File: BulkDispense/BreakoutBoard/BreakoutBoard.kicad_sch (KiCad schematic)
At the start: 30 parts, among them J1 PS, J10 R0~R5, J11 WL1, J12 WL2, J13 DigitalOUT 0~3, J14 DigitalOUT 4~7, J15 WB1, J16 WB2, J17 AnalogIOs, J18 WB-MV1&2, J19 WB-MV3&4, J2 MV1&2, J20 FS1, J21 FS2~FS4, J22 WB-MV5&6, J24 LDS, J3 MV3&4, J4 RV1~4, J5 PCV, J6 FS1, J7 FS3, J8 FS2, J9 FS4

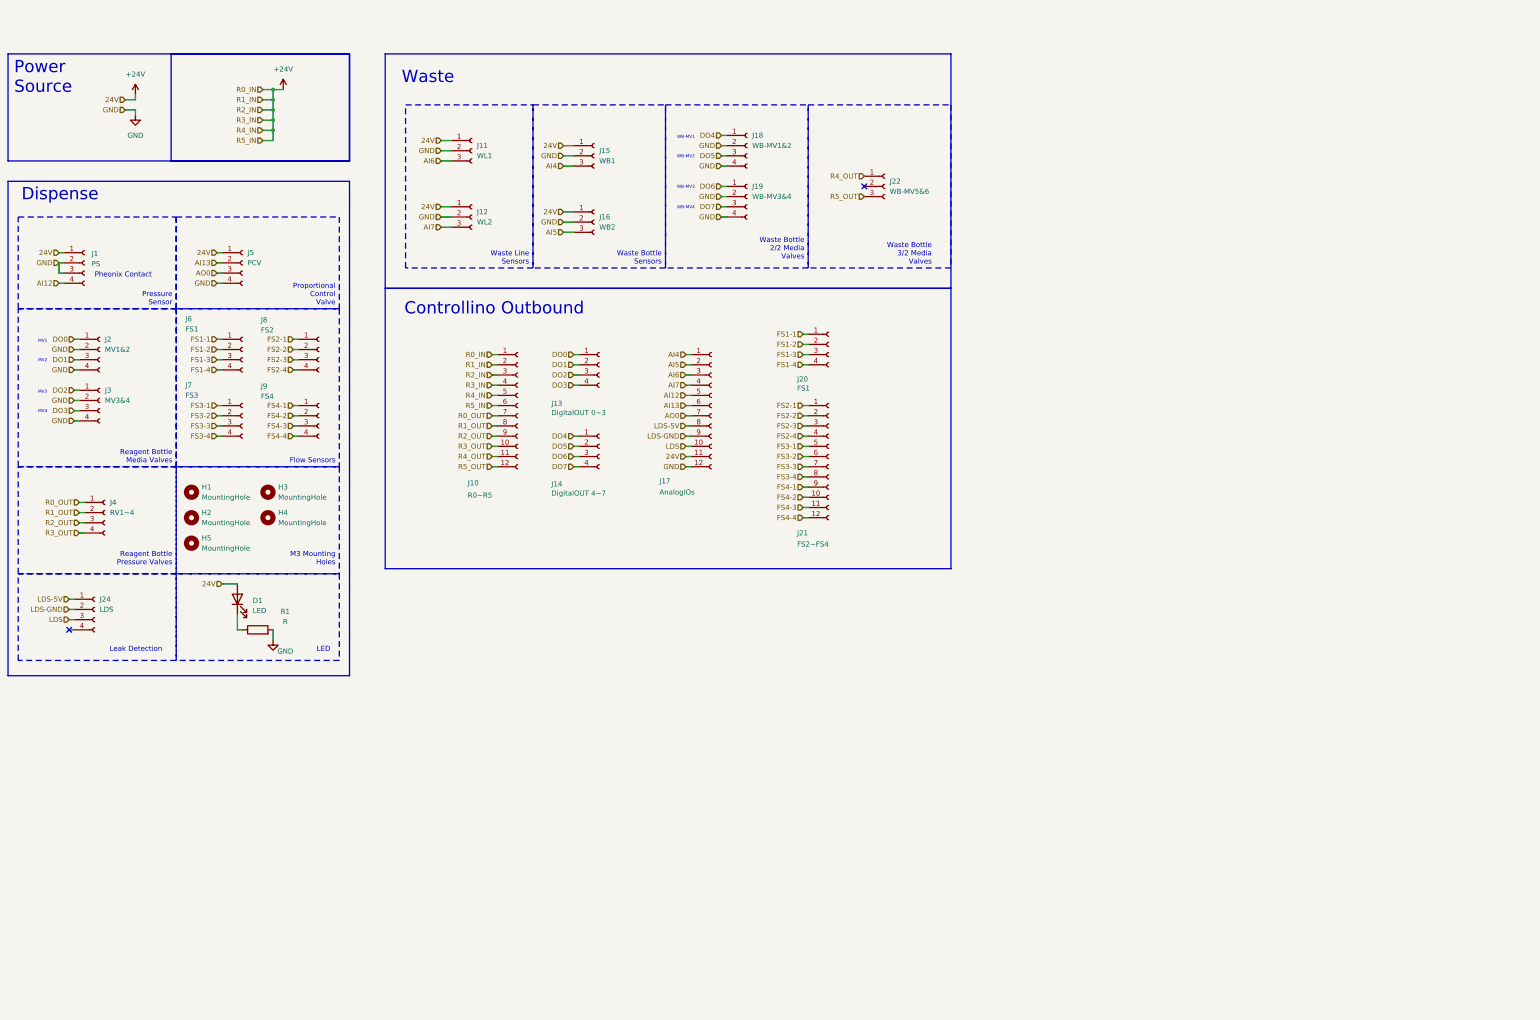
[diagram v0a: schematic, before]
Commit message: Add New Design
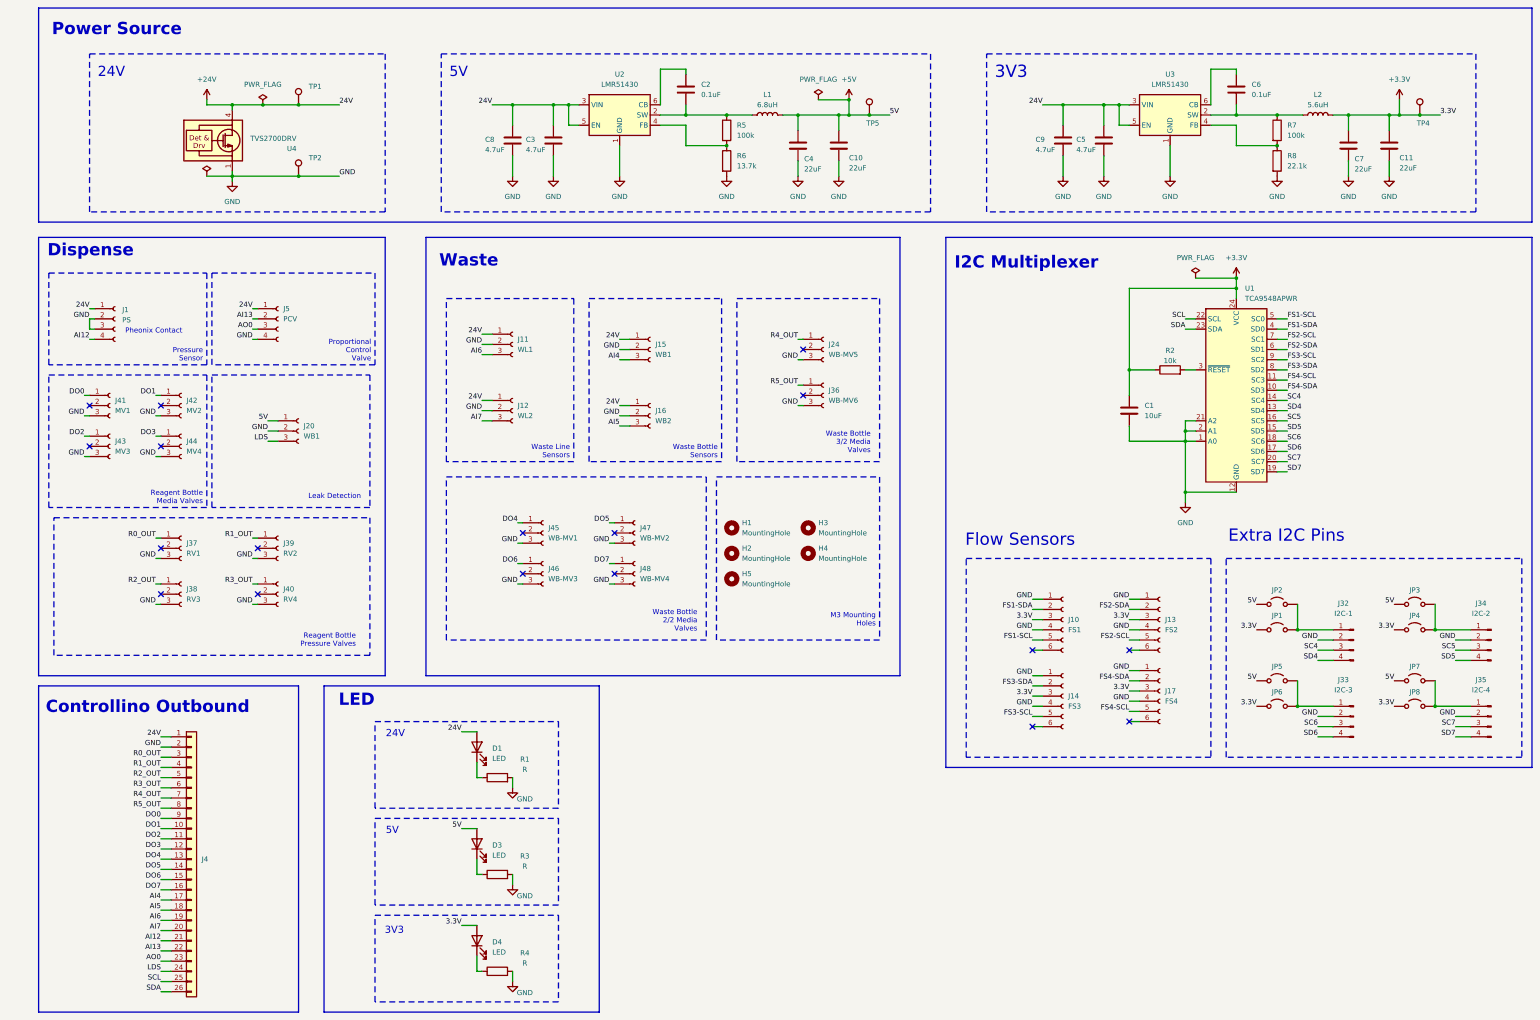
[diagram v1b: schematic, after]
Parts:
- removed J10: R0~R5, PartsLibrary:CONN_37212-62M3-003PL_3MM, symbol Connector:Conn_01x12_Socket
- removed J13: DigitalOUT 0~3, PartsLibrary:CONN_37204-62A3-004PL_3MM, symbol Connector:Conn_01x04_Socket
- removed J14: DigitalOUT 4~7, PartsLibrary:CONN_37204-62A3-004PL_3MM, symbol Connector:Conn_01x04_Socket
- removed J17: AnalogIOs, PartsLibrary:CONN_37212-62M3-003PL_3MM, symbol Connector:Conn_01x12_Socket
- removed J18: WB-MV1&2, PartsLibrary:CONN_37204-62A3-004PL_3MM, symbol Connector:Conn_01x04_Socket
- removed J19: WB-MV3&4, PartsLibrary:CONN_37204-62A3-004PL_3MM, symbol Connector:Conn_01x04_Socket
- removed J2: MV1&2, PartsLibrary:CONN_37204-62A3-004PL_3MM, symbol Connector:Conn_01x04_Socket
- removed J20, J6: FS1, PartsLibrary:CONN_37204-62A3-004PL_3MM, symbol Connector:Conn_01x04_Socket
- removed J21: FS2~FS4, PartsLibrary:CONN_37212-62M3-003PL_3MM, symbol Connector:Conn_01x12_Socket
- removed J22: WB-MV5&6, PartsLibrary:CONN_37203-62A3-003PL_3MM, symbol Connector:Conn_01x03_Socket
- removed J24: LDS, PartsLibrary:CONN_37204-62A3-004PL_3MM, symbol Connector:Conn_01x04_Socket
- removed J3: MV3&4, PartsLibrary:CONN_37204-62A3-004PL_3MM, symbol Connector:Conn_01x04_Socket
- removed J4: RV1~4, PartsLibrary:CONN_37204-62A3-004PL_3MM, symbol Connector:Conn_01x04_Socket
- removed J7: FS3, PartsLibrary:CONN_37204-62A3-004PL_3MM, symbol Connector:Conn_01x04_Socket
- removed J8: FS2, PartsLibrary:CONN_37204-62A3-004PL_3MM, symbol Connector:Conn_01x04_Socket
- removed J9: FS4, PartsLibrary:CONN_37204-62A3-004PL_3MM, symbol Connector:Conn_01x04_Socket
- added C1: 10uF, symbol Device:C
- added C10, C11, C4, C7: 22uF, symbol Device:C
- added C2, C6: 0.1uF, symbol Device:C
- added C3, C5, C8, C9: 4.7uF, symbol Device:C
- added D3, D4: LED, LED_SMD:LED_0201_0603Metric, symbol Device:LED
- added J10: FS1, symbol Connector:Conn_01x06_Socket
- added J13: FS2, symbol Connector:Conn_01x06_Socket
- added J14: FS3, symbol Connector:Conn_01x06_Socket
- added J17: FS4, symbol Connector:Conn_01x06_Socket
- added J20: WB1, PartsLibrary:CONN_37203-62A3-003PL_3MM, symbol Connector:Conn_01x03_Socket
- added J24: WB-MV5, PartsLibrary:CONN_37203-62A3-003PL_3MM, symbol Connector:Conn_01x03_Socket
- added J32: I2C-1, symbol Connector:Conn_01x04_Pin
- added J33: I2C-3, symbol Connector:Conn_01x04_Pin
- added J34: I2C-2, symbol Connector:Conn_01x04_Pin
- added J35: I2C-4, symbol Connector:Conn_01x04_Pin
- added J36: WB-MV6, PartsLibrary:CONN_37203-62A3-003PL_3MM, symbol Connector:Conn_01x03_Socket
- added J37: RV1, PartsLibrary:CONN_37203-62A3-003PL_3MM, symbol Connector:Conn_01x03_Socket
- added J38: RV3, PartsLibrary:CONN_37203-62A3-003PL_3MM, symbol Connector:Conn_01x03_Socket
- added J39: RV2, PartsLibrary:CONN_37203-62A3-003PL_3MM, symbol Connector:Conn_01x03_Socket
- added J4: Signal, PartsLibrary:CONN26_D13-ST-BK_SUL, symbol Connector_Generic:Conn_01x26
- added J40: RV4, PartsLibrary:CONN_37203-62A3-003PL_3MM, symbol Connector:Conn_01x03_Socket
- added J41: MV1, PartsLibrary:CONN_37203-62A3-003PL_3MM, symbol Connector:Conn_01x03_Socket
- added J42: MV2, PartsLibrary:CONN_37203-62A3-003PL_3MM, symbol Connector:Conn_01x03_Socket
- added J43: MV3, PartsLibrary:CONN_37203-62A3-003PL_3MM, symbol Connector:Conn_01x03_Socket
- added J44: MV4, PartsLibrary:CONN_37203-62A3-003PL_3MM, symbol Connector:Conn_01x03_Socket
- added J45: WB-MV1, PartsLibrary:CONN_37203-62A3-003PL_3MM, symbol Connector:Conn_01x03_Socket
- added J46: WB-MV3, PartsLibrary:CONN_37203-62A3-003PL_3MM, symbol Connector:Conn_01x03_Socket
- added J47: WB-MV2, PartsLibrary:CONN_37203-62A3-003PL_3MM, symbol Connector:Conn_01x03_Socket
- added J48: WB-MV4, PartsLibrary:CONN_37203-62A3-003PL_3MM, symbol Connector:Conn_01x03_Socket
- added JP1, JP2, JP3, JP4, JP5, JP6, JP7, JP8: Jumper_2_Open, Connector_PinHeader_1.00mm:PinHeader_1x02_P1.00mm_Vertical, symbol Jumper:Jumper_2_Open
- added L1: 6.8uH, symbol Device:L
- added L2: 5.6uH, symbol Device:L
- added R2: 10k, symbol Device:R
- added R3, R4: R, Resistor_SMD:R_0805_2012Metric, symbol Device:R
- added R5, R7: 100k, symbol Device:R
- added R6: 13.7k, symbol Device:R
- added R8: 22.1k, symbol Device:R
- added TP1, TP2, TP4, TP5: TestPoint, symbol Connector:TestPoint
- added U1: TCA9548APWR, Package_SO:TSSOP-24_4.4x7.8mm_P0.65mm, symbol Interface_Expansion:TCA9548APWR
- added U2, U3: LMR51430, Package_TO_SOT_SMD:SOT-23-6, symbol Regulator_Switching:LMR51430
- added U4: TVS2700DRV, Package_SON:WSON-6-1EP_2x2mm_P0.65mm_EP1x1.6mm, symbol Power_Protection:TVS2700DRV
- D1: footprint LED_SMD:LED_1206_3216Metric -> LED_SMD:LED_0201_0603Metric
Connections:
- net +24V: now also C3.1, C5.1, C8.1, C9.1, J4.1 (Pin_1), TP1.1, U2.3 (VIN), U2.5 (EN), U3.3 (VIN), U3.5 (EN), U4.4 (IN), U4.5 (IN), U4.6 (IN)
- net AI12: now also J4.21 (Pin_21)
- net AI13: now also J4.22 (Pin_22)
- net AI4: now also J4.17 (Pin_17)
- net AI5: now also J4.18 (Pin_18)
- net AI6: now also J4.19 (Pin_19)
- net AI7: now also J4.20 (Pin_20)
- net AO0: now also J4.23 (Pin_23)
- net DO0: now also J4.9 (Pin_9), J41.1 (Pin_1)
- net DO1: now also J4.10 (Pin_10), J42.1 (Pin_1)
- net DO2: now also J4.11 (Pin_11), J43.1 (Pin_1)
- net DO3: now also J4.12 (Pin_12), J44.1 (Pin_1)
- net DO4: now also J4.13 (Pin_13), J45.1 (Pin_1)
- net DO5: now also J4.14 (Pin_14), J47.1 (Pin_1)
- net DO6: now also J4.15 (Pin_15), J46.1 (Pin_1)
- net DO7: now also J4.16 (Pin_16), J48.1 (Pin_1)
- net GND: now also C1.2, C10.2, C11.2, C3.2, C4.2, C5.2, C7.2, C8.2, C9.2, J10.1 (Pin_1), J10.4 (Pin_4), J13.1 (Pin_1), J13.4 (Pin_4), J14.1 (Pin_1), J14.4 (Pin_4), J17.1 (Pin_1), J17.4 (Pin_4), J20.2 (Pin_2), J24.3 (Pin_3), J32.2 (Pin_2), J33.2 (Pin_2), J34.2 (Pin_2), J35.2 (Pin_2), J36.3 (Pin_3), J37.3 (Pin_3), J38.3 (Pin_3), J39.3 (Pin_3), J4.2 (Pin_2), J40.3 (Pin_3), J41.3 (Pin_3), J42.3 (Pin_3), J43.3 (Pin_3), J44.3 (Pin_3), J45.3 (Pin_3), J46.3 (Pin_3), J47.3 (Pin_3), J48.3 (Pin_3), R3.2, R4.2, R6.2, R8.2, TP2.1, U1.1 (A0), U1.12 (GND), U1.2 (A1), U1.21 (A2), U2.1 (GND), U3.1 (GND), U4.1 (GND), U4.2 (GND), U4.3 (GND), U4.7 (GND)
- net LDS: now also J20.3 (Pin_3), J4.24 (Pin_24)
- net R0_OUT: now also J37.1 (Pin_1), J4.3 (Pin_3)
- net R1_OUT: now also J39.1 (Pin_1), J4.4 (Pin_4)
- net R2_OUT: now also J38.1 (Pin_1), J4.5 (Pin_5)
- net R3_OUT: now also J4.6 (Pin_6), J40.1 (Pin_1)
- net R4_OUT: now also J24.1 (Pin_1), J4.7 (Pin_7)
- net R5_OUT: now also J36.1 (Pin_1), J4.8 (Pin_8)
- new net: J33.1 (Pin_1), JP5.2 (B), JP6.2 (B)
- new net: C2.1, U2.6 (CB)
- new net: C2.2, L1.1, R5.1, U2.2 (SW)
- new net: J35.1 (Pin_1), JP7.2 (B), JP8.2 (B)
- new net: J34.1 (Pin_1), JP3.2 (B), JP4.2 (B)
- new net: J32.1 (Pin_1), JP1.2 (B), JP2.2 (B)
- new net: C6.1, U3.6 (CB)
- new net: C6.2, L2.1, R7.1, U3.2 (SW)
- new net: D4.1 (K), R4.1
- new net: R7.2, R8.1, U3.4 (FB)
- new net: R2.2, U1.3 (~{RESET})
- new net: R5.2, R6.1, U2.4 (FB)
- new net: D3.1 (K), R3.1
- new net +3.3V: C1.1, C11.1, C7.1, D4.2 (A), J10.3 (Pin_3), J13.3 (Pin_3), J14.3 (Pin_3), J17.3 (Pin_3), JP1.1 (A), JP4.1 (A), JP6.1 (A), JP8.1 (A), L2.2, R2.1, TP4.1, U1.24 (VCC)
- new net +5V: C10.1, C4.1, D3.2 (A), J20.1 (Pin_1), JP2.1 (A), JP3.1 (A), JP5.1 (A), JP7.1 (A), L1.2, TP5.1
- new net FS1-SCL: J10.5 (Pin_5), U1.5 (SC0)
- new net FS1-SDA: J10.2 (Pin_2), U1.4 (SD0)
- new net FS2-SCL: J13.5 (Pin_5), U1.7 (SC1)
- new net FS2-SDA: J13.2 (Pin_2), U1.6 (SD1)
- new net FS3-SCL: J14.5 (Pin_5), U1.9 (SC2)
- new net FS3-SDA: J14.2 (Pin_2), U1.8 (SD2)
- new net FS4-SCL: J17.5 (Pin_5), U1.11 (SC3)
- new net FS4-SDA: J17.2 (Pin_2), U1.10 (SD3)
- new net SC4: J32.3 (Pin_3), U1.14 (SC4)
- new net SC5: J34.3 (Pin_3), U1.16 (SC5)
- new net SC6: J33.3 (Pin_3), U1.18 (SC6)
- new net SC7: J35.3 (Pin_3), U1.20 (SC7)
- new net SCL: J4.25 (Pin_25), U1.22 (SCL)
- new net SD4: J32.4 (Pin_4), U1.13 (SD4)
- new net SD5: J34.4 (Pin_4), U1.15 (SD5)
- new net SD6: J33.4 (Pin_4), U1.17 (SD6)
- new net SD7: J35.4 (Pin_4), U1.19 (SD7)
- new net SDA: J4.26 (Pin_26), U1.23 (SDA)
- no-connect marks 2 -> 18
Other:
- note added: "24V"
- note added: "3V3"
- note added: "5V"
- note added: "Extra I2C Pins"
- note added: "Flow Sensors"
- note added: "I2C Multiplexer"
- note added: "LED"
- note removed: "MV1"
- note removed: "MV2"
- note removed: "MV3"
- note removed: "MV4"
- note removed: "WB-MV1"
- note removed: "WB-MV2"
- note removed: "WB-MV3"
- note removed: "WB-MV4"
- moved on the sheet: D1, H1, H2, H3, H4, H5, J1, J11, J12, J15, J16, J5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
